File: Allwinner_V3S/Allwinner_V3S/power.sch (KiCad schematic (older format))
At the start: 22 parts, among them U2 SY8088AAC, U3 SY8088AAC, U4 SY8088AAC

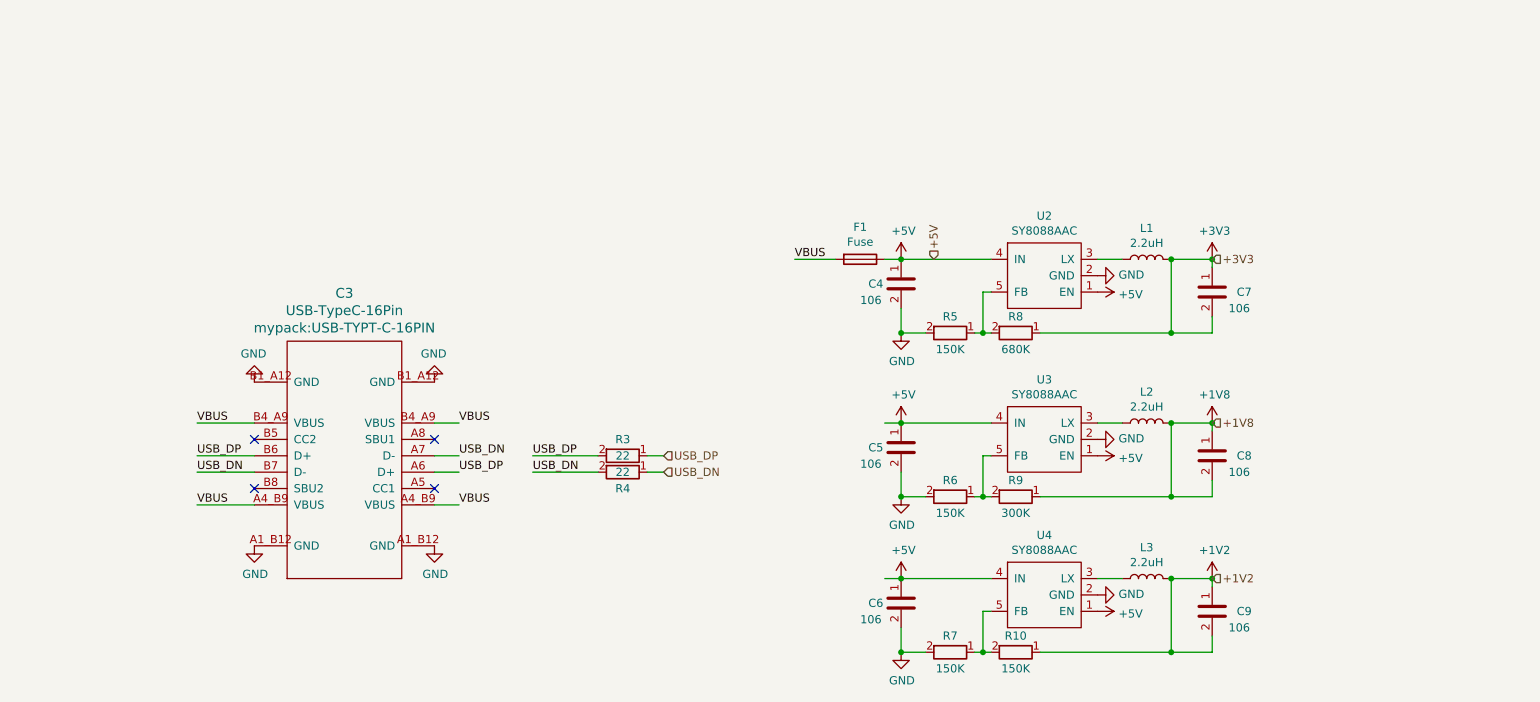
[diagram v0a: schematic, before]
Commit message: update
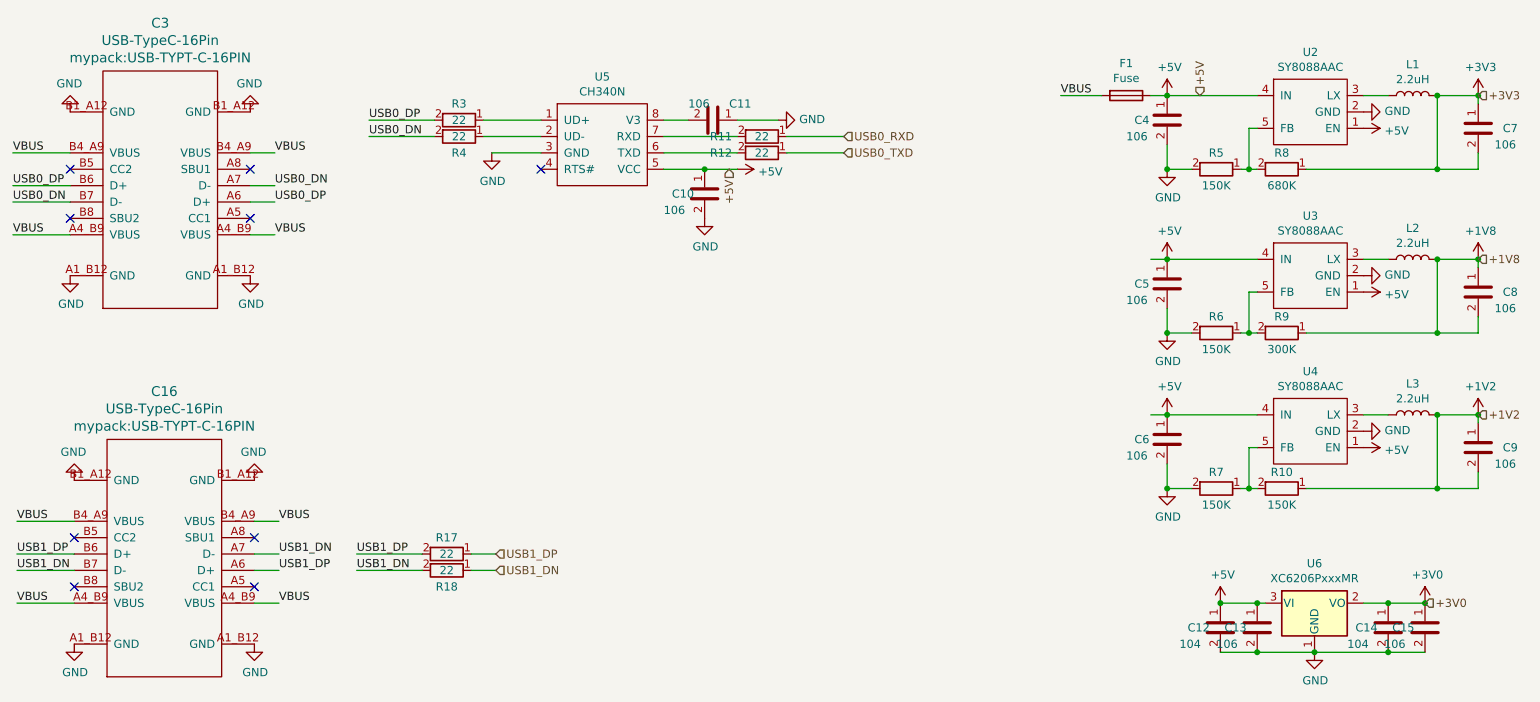
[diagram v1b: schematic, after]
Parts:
- added C10, C11, C13, C15: 106, Capacitor_SMD:C_0402_1005Metric, symbol mylib:C_0402
- added C12, C14: 104, Capacitor_SMD:C_0402_1005Metric, symbol mylib:C_0402
- added C16: USB-TypeC-16Pin, mypack:USB-TYPT-C-16PIN, symbol mylib:USB-TypeC-16Pin
- added R11, R12, R17, R18: 22, Resistor_SMD:R_0402_1005Metric, symbol mylib:R_0402
- added U5: CH340N, Package_SO:SOP-8_3.9x4.9mm_P1.27mm, symbol mylib:CH340N
- added U6: XC6206PxxxMR, Package_TO_SOT_SMD:SOT-23, symbol Regulator_Linear:XC6206PxxxMR
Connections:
- net labels added: +3V0, USB0_DN, USB0_DP, USB0_RXD, USB0_TXD, USB1_DN, USB1_DP
- net labels removed: USB_DN, USB_DP
- wire segments 58 -> 87
- no-connect marks 4 -> 9
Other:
- moved on the sheet: C3, C4, C5, C6, C7, C8, C9, F1, L1, L2, L3, R10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
